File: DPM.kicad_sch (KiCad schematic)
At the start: 15 parts, among them J1 Conn_01x08, U1 74HC590, U2 74HC682, U4 MCP23017_SP

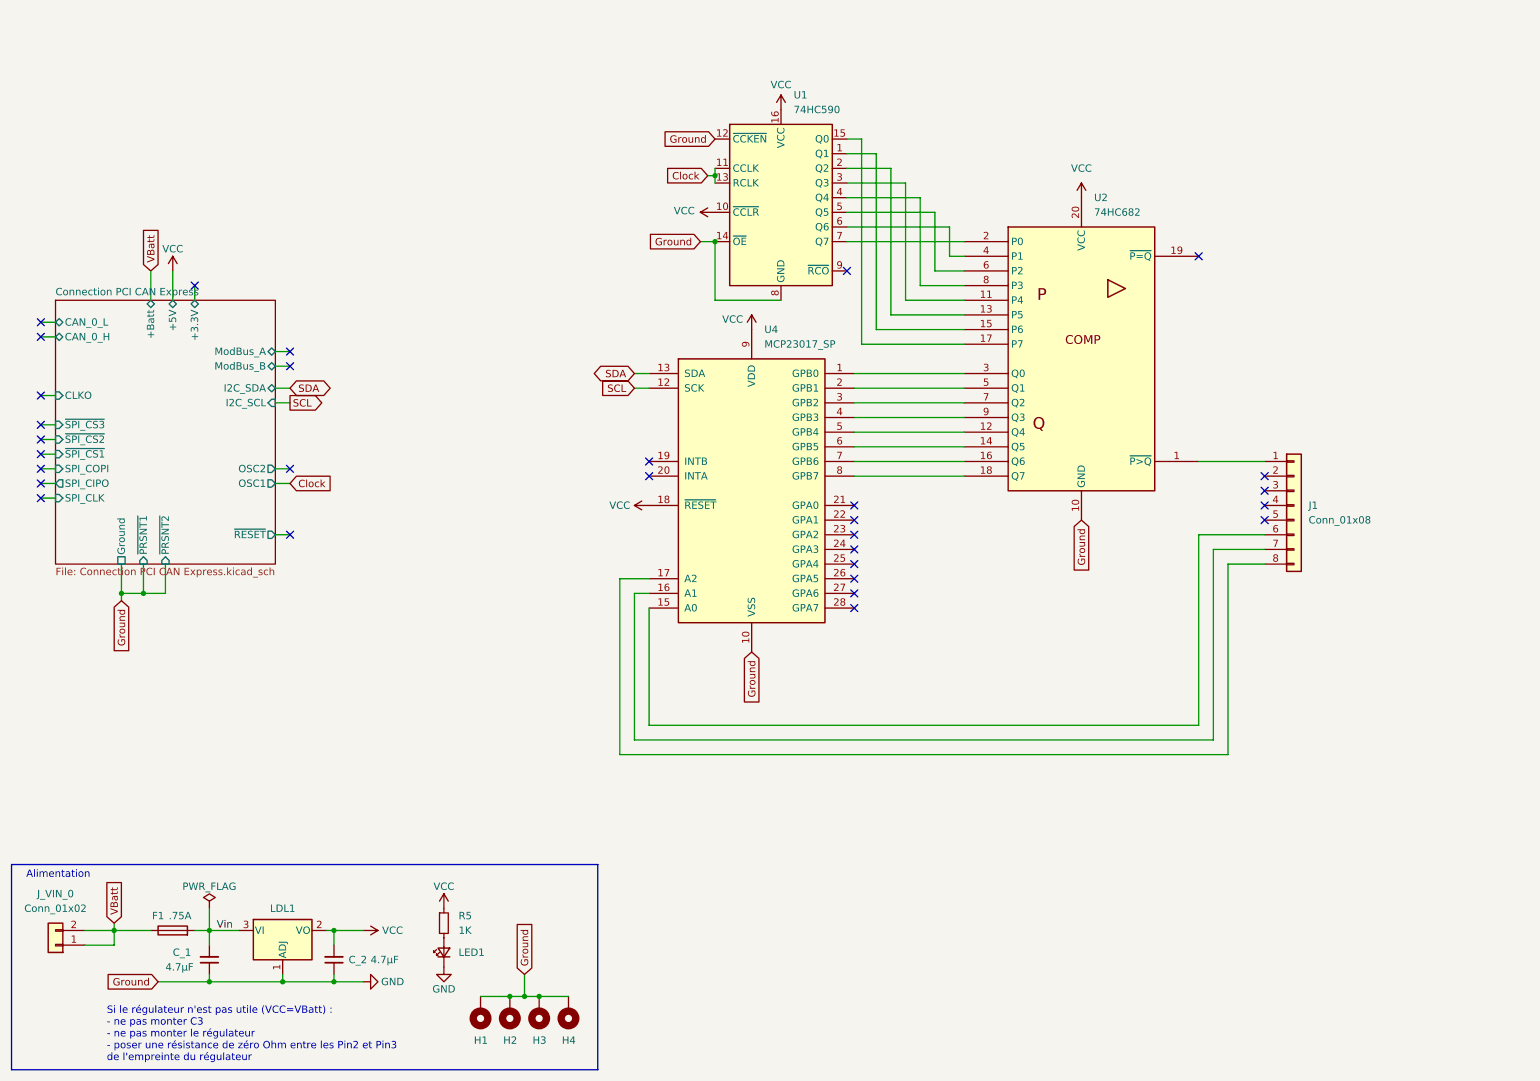
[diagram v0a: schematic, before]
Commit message: DPM et DDPM implémentés Mouais bof pour ajouter ma DPM en code Gray
Sinon OK Tiers pour en faire la branche 1

git-svn-id: file:///D%5C00%20-%20Dev%20&%20Calculs%5CRepoTortoiseSVN_PCB%5CD-DPM/trunk@14 f29d8339-a183-0348-962e-9e4594cf8312
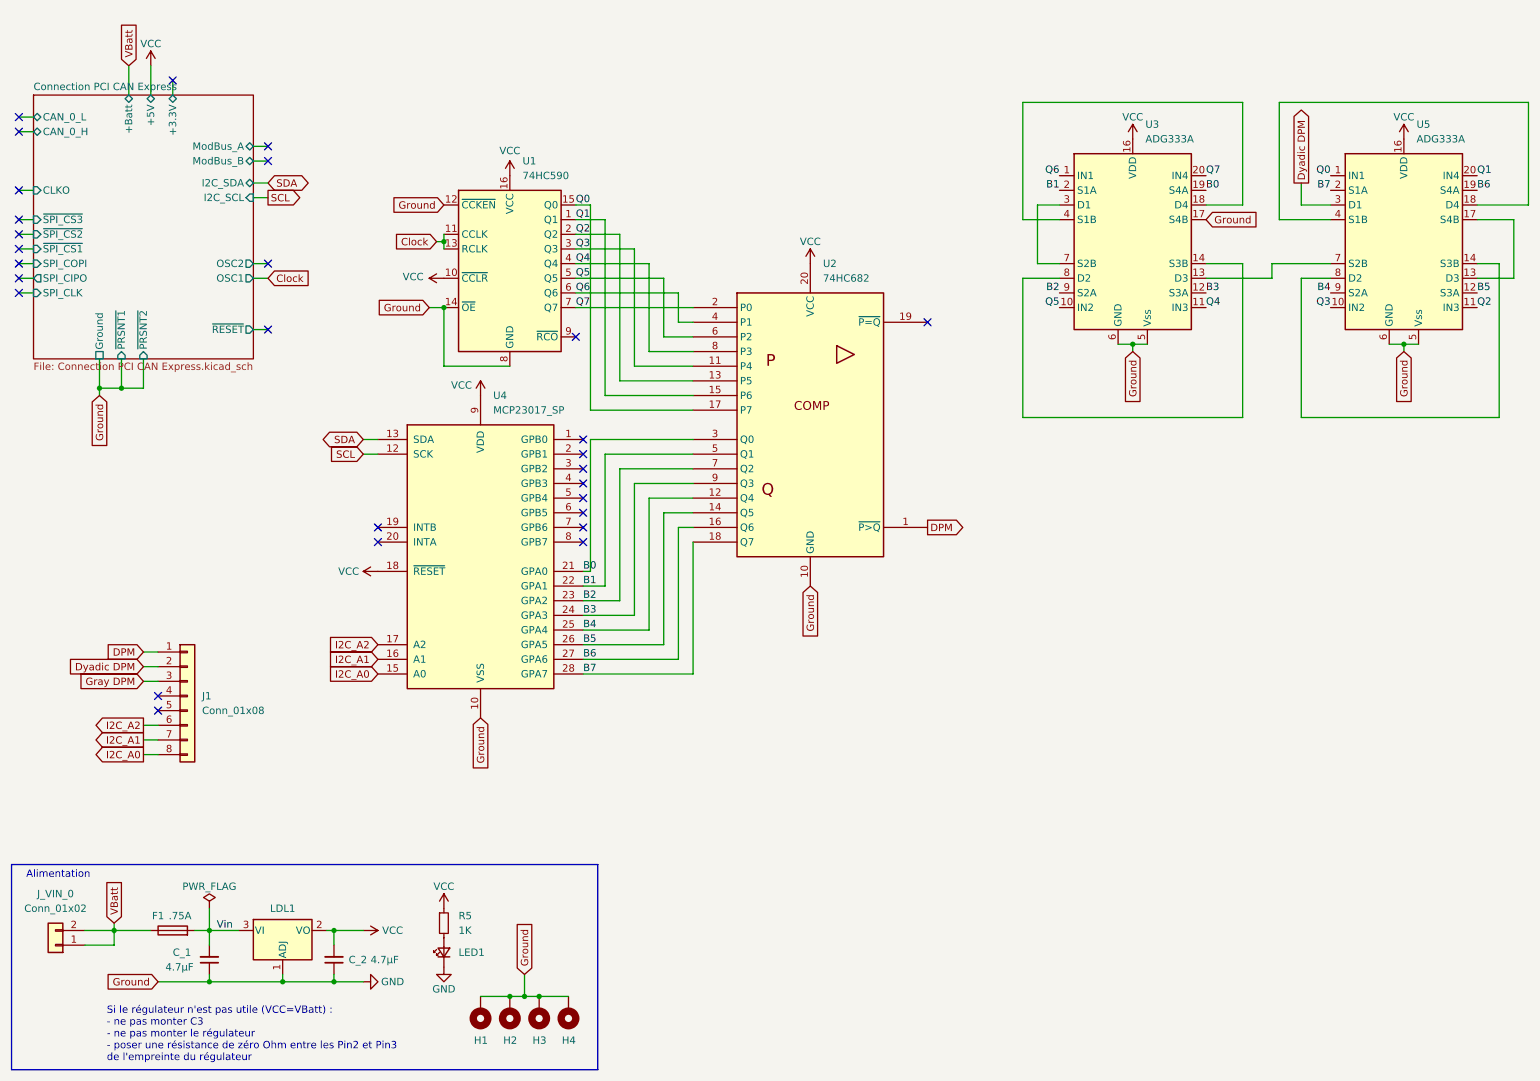
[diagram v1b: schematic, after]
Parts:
- added U3, U5: ADG333A, Package_DIP:DIP-20_W7.62mm_Socket_LongPads, symbol Perso_Spare_parts:ADG333A
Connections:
- net GND: now also U3.15 (NC), U3.17 (S4B), U3.5 (Vss), U3.6 (GND), U5.15 (NC), U5.5 (Vss), U5.6 (GND)
- net VCC: now also U3.16 (VDD), U5.16 (VDD)
- net DPM: now reaches J1.1 (Pin_1), U2.1 (~{P>Q})
- net Dyadic DPM: now reaches J1.2 (Pin_2)
- net Dyadic DPM: now also U5.3 (D1)
- net Gray DPM: now reaches J1.3 (Pin_3)
- net I2C_A0: now reaches U4.15 (A0)
- net I2C_A0: now also J1.8 (Pin_8); no longer J1.6 (Pin_6)
- net I2C_A1: now reaches J1.7 (Pin_7), U4.16 (A1)
- net I2C_A2: now reaches U4.17 (A2)
- net I2C_A2: now also J1.6 (Pin_6); no longer J1.8 (Pin_8)
- net Q1: now reaches U1.1 (Q1), U2.15 (P6)
- net Q1: now also U5.20 (IN4)
- net Q0: now reaches U1.15 (Q0), U2.17 (P7)
- net Q0: now also U5.1 (IN1)
- net Q2: now reaches U1.2 (Q2), U2.13 (P5)
- net Q2: now also U5.11 (IN3)
- net Q3: now reaches U1.3 (Q3), U2.11 (P4)
- net Q3: now also U5.10 (IN2)
- net Q4: now reaches U1.4 (Q4), U2.8 (P3)
- net Q4: now also U3.11 (IN3)
- net Q5: now reaches U1.5 (Q5), U2.6 (P2)
- net Q5: now also U3.10 (IN2)
- net Q6: now reaches U1.6 (Q6), U2.4 (P1)
- net Q6: now also U3.1 (IN1)
- net Q7: now reaches U1.7 (Q7), U2.2 (P0)
- net Q7: now also U3.20 (IN4)
- net at U4.1 (GPB0): no longer U2.3 (Q0)
- net at U4.2 (GPB1): no longer U2.5 (Q1)
- net B0: now reaches U4.21 (GPA0)
- net B0: now also U2.3 (Q0), U3.19 (S4A)
- net B1: now reaches U4.22 (GPA1)
- net B1: now also U2.5 (Q1), U3.2 (S1A)
- net B2: now reaches U4.23 (GPA2)
- net B2: now also U2.7 (Q2), U3.9 (S2A)
- net B3: now reaches U4.24 (GPA3)
- net B3: now also U2.9 (Q3), U3.12 (S3A)
- net B4: now reaches U4.25 (GPA4)
- net B4: now also U2.12 (Q4), U5.9 (S2A)
- net B5: now reaches U4.26 (GPA5)
- net B5: now also U2.14 (Q5), U5.12 (S3A)
- net B6: now reaches U4.27 (GPA6)
- net B6: now also U2.16 (Q6), U5.19 (S4A)
- net B7: now reaches U4.28 (GPA7)
- net B7: now also U2.18 (Q7), U5.2 (S1A)
- net at U4.3 (GPB2): no longer U2.7 (Q2)
- net at U4.4 (GPB3): no longer U2.9 (Q3)
- net at U4.5 (GPB4): no longer U2.12 (Q4)
- net at U4.6 (GPB5): no longer U2.14 (Q5)
- net at U4.7 (GPB6): no longer U2.16 (Q6)
- net at U4.8 (GPB7): no longer U2.18 (Q7)
- new net: U5.13 (D3), U5.17 (S4B)
- new net: U5.14 (S3B), U5.8 (D2)
- new net: U5.18 (D4), U5.4 (S1B)
- new net: U3.13 (D3), U5.7 (S2B)
- new net: U3.14 (S3B), U3.8 (D2)
- new net: U3.18 (D4), U3.4 (S1B)
- new net: U3.3 (D1), U3.7 (S2B)
- no-connect marks 30 -> 28
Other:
- moved on the sheet: J1, U1, U2, U4
